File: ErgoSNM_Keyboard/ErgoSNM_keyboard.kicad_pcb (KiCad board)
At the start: 2 copper layers, 96 parts, among them J1 Conn_01x13, J2 Conn_01x13, J3 Conn_01x03, J4 Conn_01x04, SW1 RESET, SW2 SW_2P2T

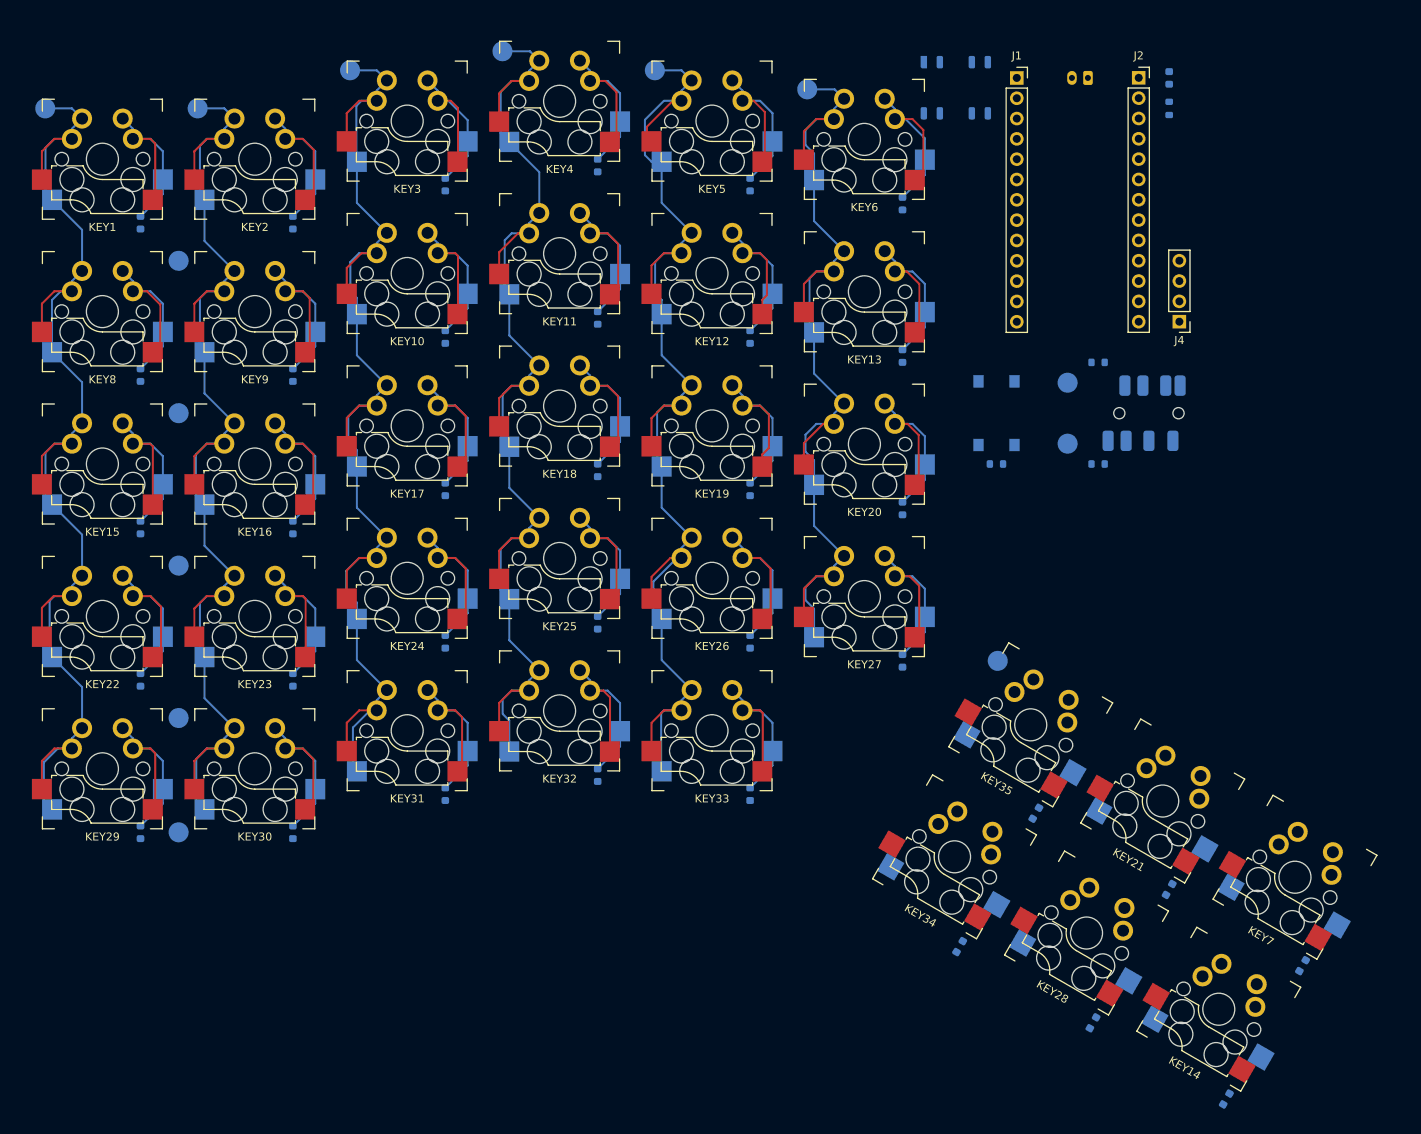
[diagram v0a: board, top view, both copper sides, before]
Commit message: Update PCB
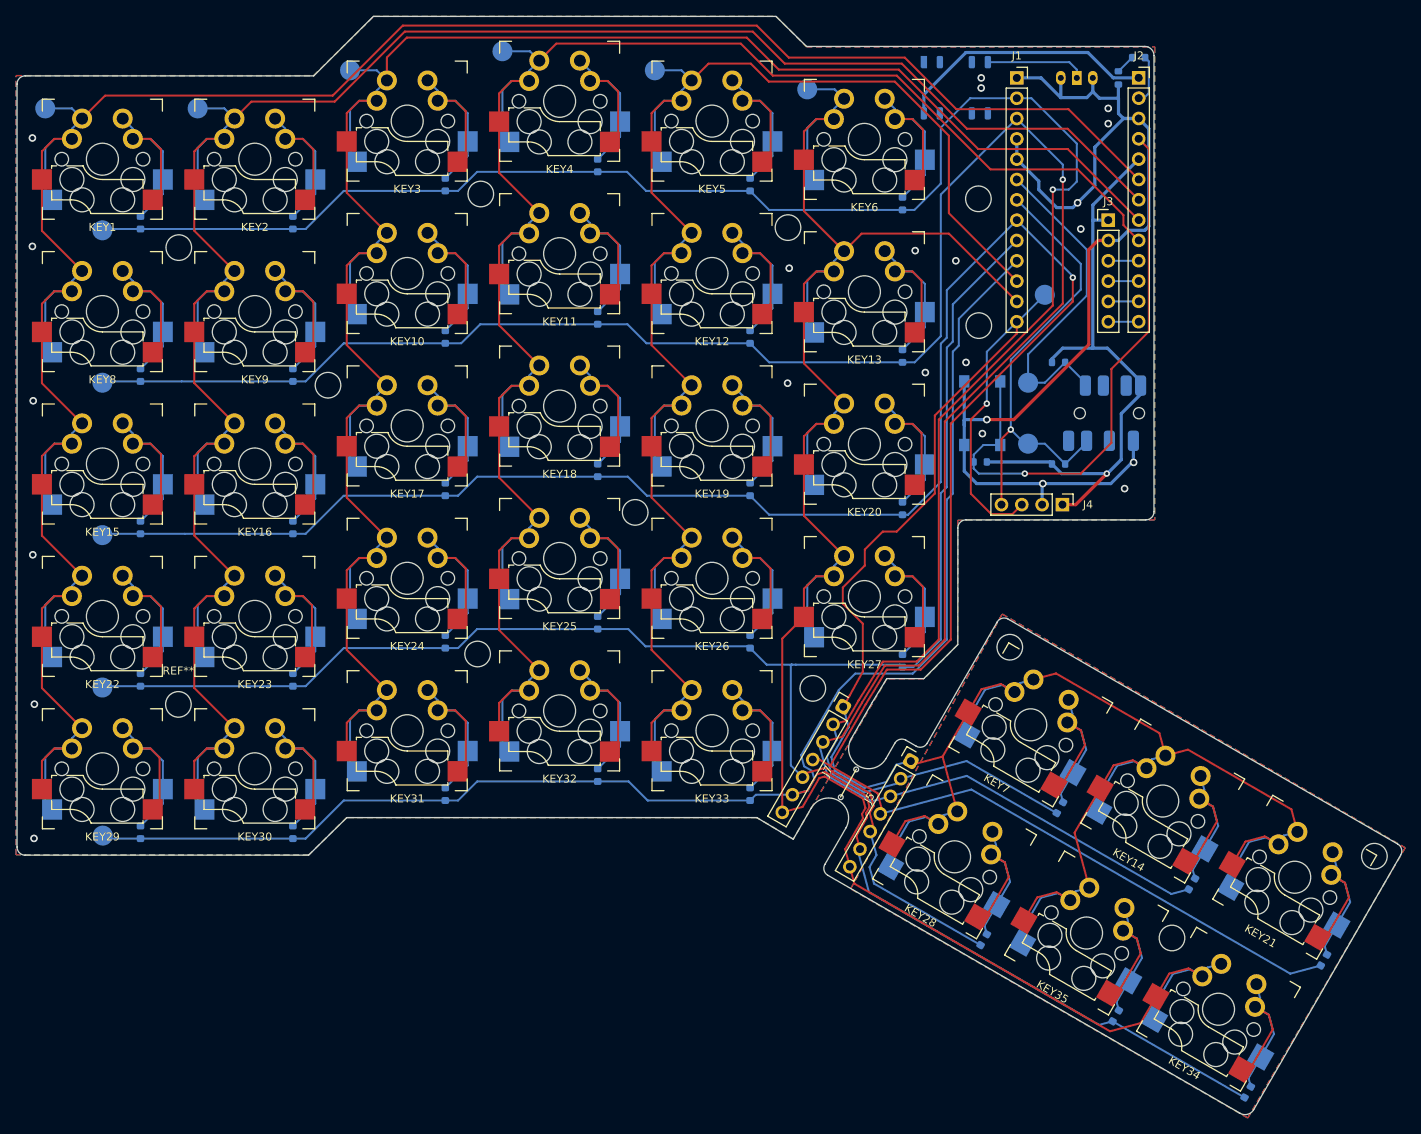
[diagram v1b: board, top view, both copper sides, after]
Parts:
- added J3: Conn_01x06, Connector_PinHeader_2.54mm:PinHeader_1x06_P2.54mm_Vertical, F.Cu at (201.9, 52.1)
- added J5: Conn_01x07, Connector_PinHeader_2.54mm:PinHeader_1x07_P2.54mm_Vertical, F.Cu at (177.3, 119.7)
- added J7: Conn_01x07, Connector_PinHeader_2.54mm:PinHeader_1x07_P2.54mm_Vertical, F.Cu at (168.8, 112.9)
- added REF**: MountingHole_3.2mm_M3, MountingHole:MountingHole_3.2mm_M3, F.Cu at (185.8, 65.2)
- added REF**: MountingHole_3.2mm_M3, MountingHole:MountingHole_3.2mm_M3, F.Cu at (185.7, 49.4)
- added REF**: MountingHole_3.2mm_M3, MountingHole:MountingHole_3.2mm_M3, F.Cu at (123.1, 106.3)
- added REF**: MountingHole_3.2mm_M3, MountingHole:MountingHole_3.2mm_M3, F.Cu at (209.9, 141.8)
- added REF**: MountingHole_3.2mm_M3, MountingHole:MountingHole_3.2mm_M3, F.Cu at (85.7, 112.6)
- added REF**: MountingHole_3.2mm_M3, MountingHole:MountingHole_3.2mm_M3, F.Cu at (170.4, 120.7)
- added REF**: MountingHole_3.2mm_M3, MountingHole:MountingHole_3.2mm_M3, F.Cu at (189.6, 105.5)
- added REF**: MountingHole_3.2mm_M3, MountingHole:MountingHole_3.2mm_M3, F.Cu at (235.2, 131.6)
- added REF**: MountingHole_3.2mm_M3, MountingHole:MountingHole_3.2mm_M3, F.Cu at (161.9, 53.0)
- added REF**: MountingHole_3.2mm_M3, MountingHole:MountingHole_3.2mm_M3, F.Cu at (85.8, 55.5)
- added REF**: MountingHole_3.2mm_M3, MountingHole:MountingHole_3.2mm_M3, F.Cu at (123.5, 48.8)
- added REF**: MountingHole_3.2mm_M3, MountingHole:MountingHole_3.2mm_M3, F.Cu at (165.0, 110.6)
- added REF**: MountingHole_3.2mm_M3, MountingHole:MountingHole_3.2mm_M3, F.Cu at (104.4, 72.7)
- added REF**: MountingHole_3.2mm_M3, MountingHole:MountingHole_3.2mm_M3, F.Cu at (168.5, 124.2)
- added REF**: MountingHole_3.2mm_M3, MountingHole:MountingHole_3.2mm_M3, F.Cu at (142.8, 88.6)
- J6: renamed from J3; footprint Connector_JST:JST_PH_B2B-PH-K_1x02_P2.00mm_Vertical -> Connector_JST:JST_PH_B3B-PH-K_1x03_P2.00mm_Vertical
- moved TP13 46.1 mm to (194.0, 61.4)
- moved D34 40.3 mm to (219.4, 161.1)
- moved KEY7 38.1 mm to (192.2, 115.2)
- moved KEY34 38.1 mm to (215.7, 150.7)
- moved D7 36.2 mm to (195.9, 125.5)
- moved D14 27.2 mm to (212.4, 135.0)
- moved D35 27.2 mm to (202.9, 151.5)
- moved J4 27.1 mm to (196.2, 87.6), turned to -90 degrees
- moved KEY14 26.9 mm to (208.7, 124.7)
- moved KEY35 26.9 mm to (199.2, 141.2)
- moved D21 21.3 mm to (228.9, 144.6)
- moved KEY28 19.1 mm to (182.7, 131.7)
- moved KEY21 19.1 mm to (225.2, 134.2)
- moved D28 17.2 mm to (186.4, 142.0)
- moved TP2 10.3 mm to (76.2, 72.4)
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- renumbered D11 to D10, D12 to D11, D13 to D12, D14 to D13, D15 to D14, D16 to D15, D17 to D16, D18 to D17, D19 to D18, D20 to D19, D21 to D20, D22 to D21, D23 to D22, D24 to D23, D25 to D24, D26 to D25, D27 to D26, D28 to D27, D29 to D28, D30 to D29, D31 to D30, D32 to D31, D33 to D32, D34 to D33, D35 to D34, D36 to D35, D9 to D8, D10 to D9, D8 to LD1, TP11 to TP10, TP12 to TP11, TP13 to TP12, TP14 to TP13, TP6 to TP14, TP5 to TP4, TP7 to TP5, TP4 to TP6, TP8 to TP7, TP9 to TP8, TP10 to TP9
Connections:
- J4 pad 1: CS -> VCC
- J4 pad 2: MOSI -> GND
- J4 pad 3: MISO -> COL_6
- J4 pad 4: SCLK -> SCL
- R3 pad 2: SDA -> SCL
- R4 pad 1: SCL -> SDA
- TP14 pad 1: SCL -> SDA
- TP6 pad 1: SDA -> SCL
- TRRS1 pad 2: SCL -> SDA
- TRRS1 pad 3: SDA -> SCL
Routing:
- net ROW_2: track 0.00 -> 307.1 mm, vias 0 -> 1
- net COL_6: track 0.00 -> 295.7 mm, vias 0 -> 1
- net ROW_1: track 0.00 -> 292.6 mm, vias 0 -> 1
- net ROW_0: track 0.00 -> 265.9 mm, vias 0 -> 1
- net ROW_4: track 0.00 -> 252.6 mm
- net ROW_3: track 0.00 -> 216.9 mm
- net COL_0: track 153.3 -> 312.2 mm
- net COL_5: track 122.7 -> 274.2 mm
- net GND: track 0.00 -> 147.4 mm, vias 0 -> 23
- net COL_1: track 154.6 -> 293.5 mm
- net COL_2: track 153.5 -> 274.6 mm
- net COL_3: track 154.6 -> 254.0 mm
- net VCC: track 0.00 -> 77.8 mm, vias 0 -> 1
- net RESET: track 0.00 -> 73.0 mm, vias 0 -> 1
- net COL_4: track 154.4 -> 225.7 mm
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- added copper zone on B.Cu, net (none)
- added copper zone on F.Cu, net (none)
- added copper zone on B.Cu, net GND
- added copper zone on F.Cu, net GND
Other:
- board outline added: 173.1 x 137.3 mm
